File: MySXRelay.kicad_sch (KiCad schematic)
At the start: 52 parts, among them K1 FH44L-1AT-L1-DC5V, U1 MIC4427, U2 BL0942, U3 BP2525X, U4 Si8642BB-B-IS1, U5 MCP1703Ax-180xxTT, U8 AP2204K-ADJ, U9 ST485E

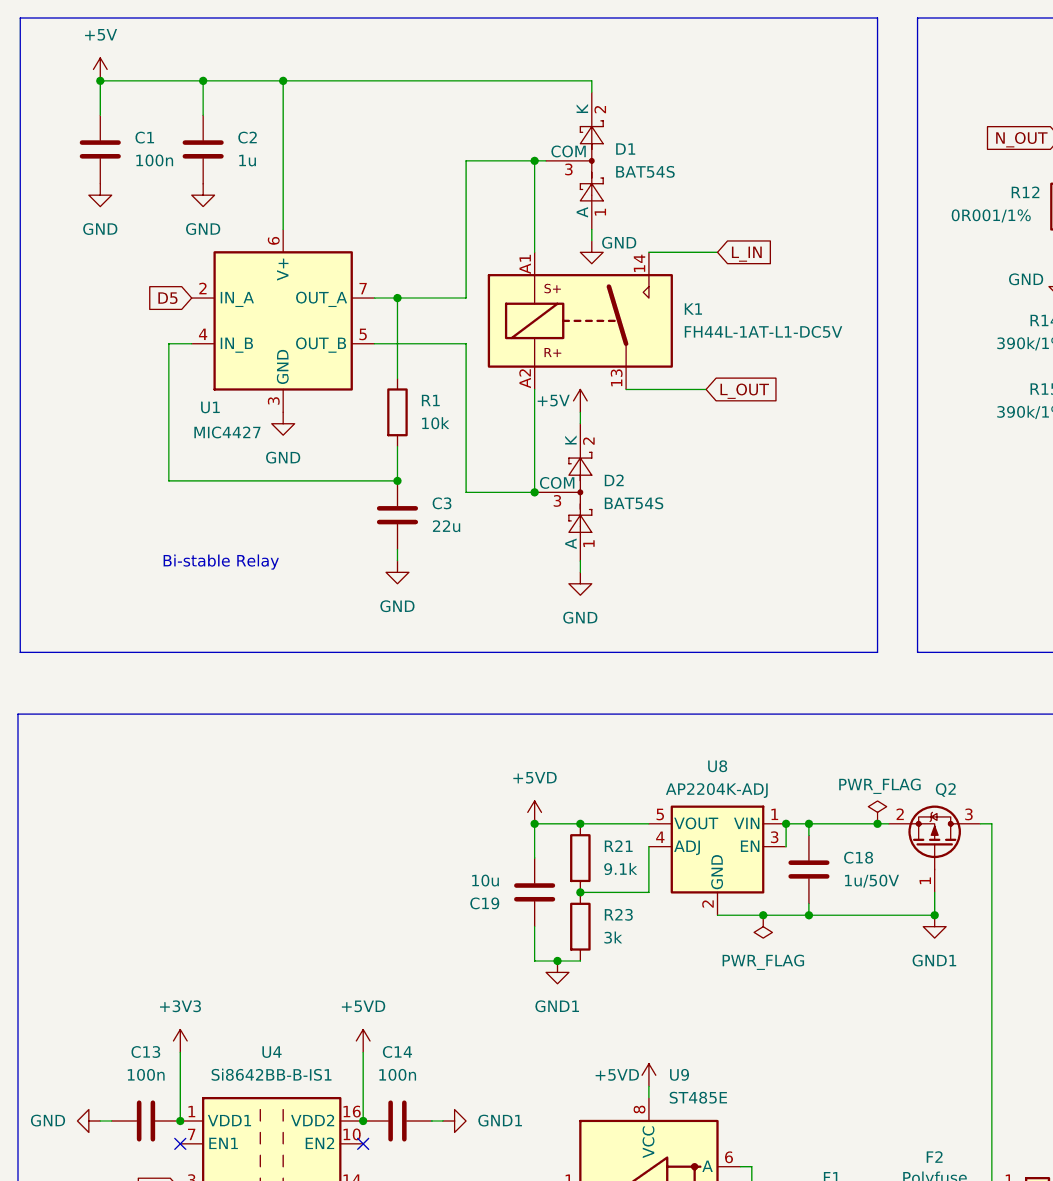
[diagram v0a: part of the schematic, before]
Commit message: update pcb (WIP)
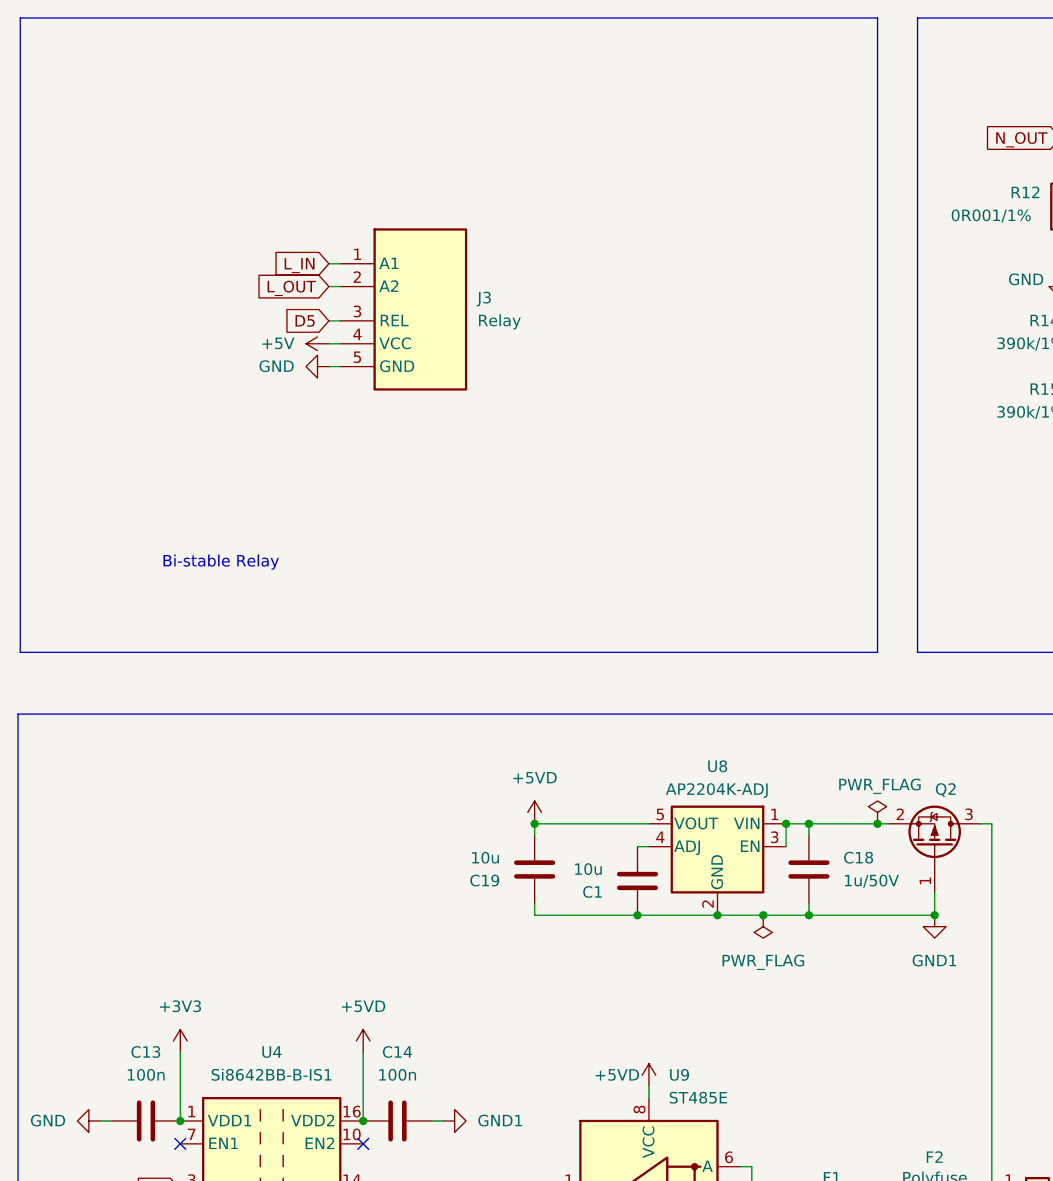
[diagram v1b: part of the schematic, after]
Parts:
- removed C2: 1u, Capacitor_SMD:C_0603_1608Metric, symbol Device:C
- removed C3: 22u, Capacitor_SMD:C_1206_3216Metric, symbol Device:C
- removed D1, D2: BAT54S, Package_TO_SOT_SMD:SOT-23, symbol Diode:BAT54S
- removed K1: FH44L-1AT-L1-DC5V, MySXRelay:RELAY-TH_FH44L-1AT-L1-DC5V, symbol MySXRelay:Relay_SPST_Latching_1coil
- removed R1: 10k, Resistor_SMD:R_0603_1608Metric, symbol Device:R
- removed R21: 9.1k, Resistor_SMD:R_0603_1608Metric, symbol Device:R
- removed R23: 3k, Resistor_SMD:R_0603_1608Metric, symbol Device:R
- removed U1: MIC4427, Package_SO:SOIC-8_3.9x4.9mm_P1.27mm, symbol Driver_FET:MIC4427
- added J3: Relay, MySXRelay:edge_connector, symbol MySXRelay:edge_connector
- C1: value 100n -> 10u; footprint Capacitor_SMD:C_0402_1005Metric -> Capacitor_SMD:C_0603_1608Metric
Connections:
- net +5V: now also J3.4 (VCC); no longer C1.1
- net D5: now also J3.3 (REL)
- net GND: now also J3.5 (GND); no longer C1.2
- net GND1: now also C1.1
- net L_IN: now also J3.1 (A1)
- net L_OUT: now also J3.2 (A2)
- net at U8.4 (ADJ): now also C1.2
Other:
- moved on the sheet: C19
